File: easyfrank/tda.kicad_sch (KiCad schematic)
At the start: 7 parts, among them U7 TDA1545A

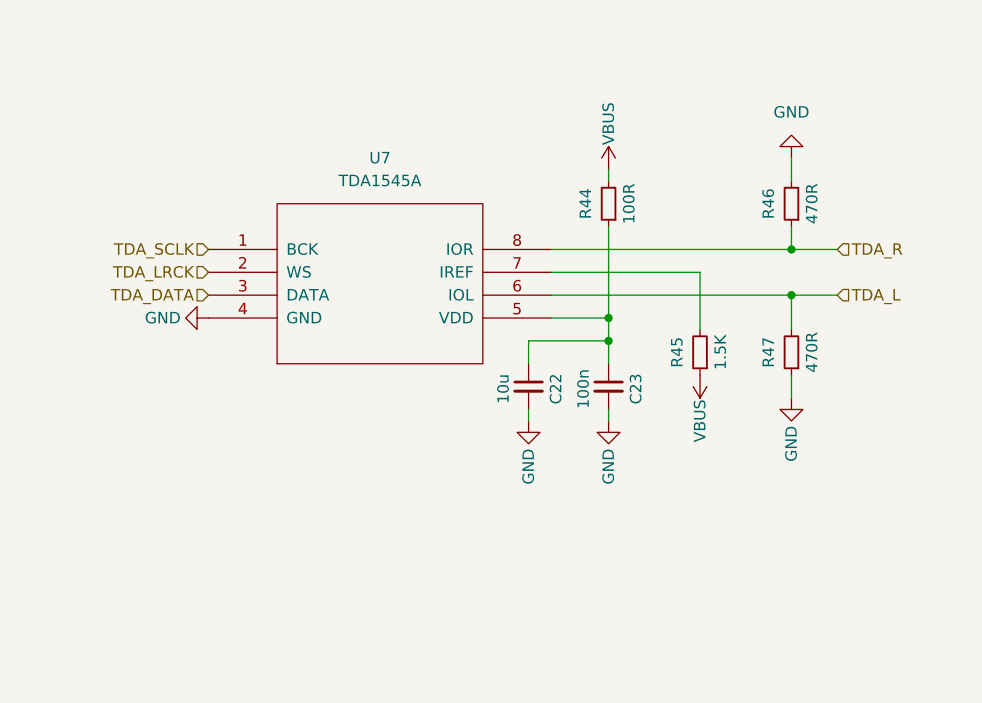
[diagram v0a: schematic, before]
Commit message: EasyFRANK WIP
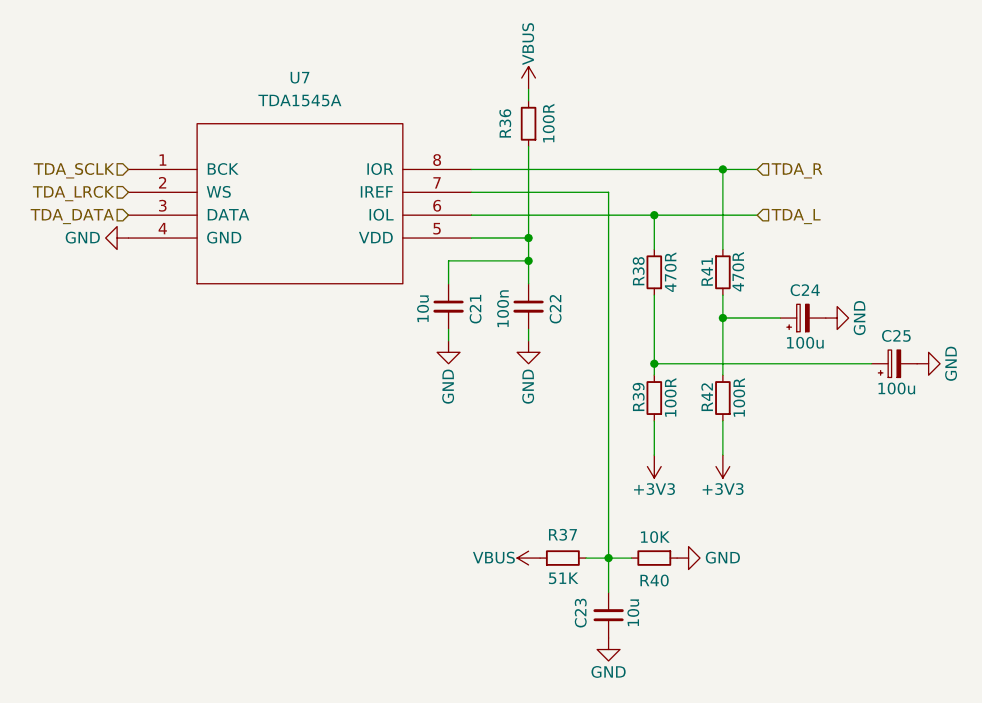
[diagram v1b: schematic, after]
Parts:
- added C23: 10u, FRANK:Combined_0805_CR, symbol FRANK:C_Small
- added C24, C25: 100u, FRANK:C_Radial_D6.3mm_P2.50mm, symbol FRANK:C_Polarized_Small
- added R37: 51K, FRANK:Combined_0805_RE, symbol FRANK:R_Small
- added R39, R42: 100R, FRANK:Combined_0805_RE, symbol FRANK:R_Small
- R40: renamed from R45; value 1.5K -> 10K
- renumbered C22 to C21, C23 to C22, R44 to R36, R47 to R38, R46 to R41
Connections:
- net GND: now also R40.1, C23.1, C24.2, C25.2; no longer R38.1, R41.2
- net VBUS: now also R37.1; no longer R40.1
- net at R40.2, U7.7 (IREF): now also C23.2, R37.2
- new net: C24.1, R41.2, R42.2
- new net: C25.1, R38.1, R39.2
- new net +3V3: R39.1, R42.1
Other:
- moved on the sheet: C21, C22, R36, R38, R40, R41, U7
